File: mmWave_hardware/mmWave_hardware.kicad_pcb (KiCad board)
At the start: 6 copper layers, 50 x 21.6 mm, 48 parts, among them J1 Conn_02x08_Top_Bottom, U1 IWRL6432BDBAAMFR, U2 W25Q128JVS, U3 AMS1117-3.3, U4 TPS628502QDRLRQ1, Y1 40.000

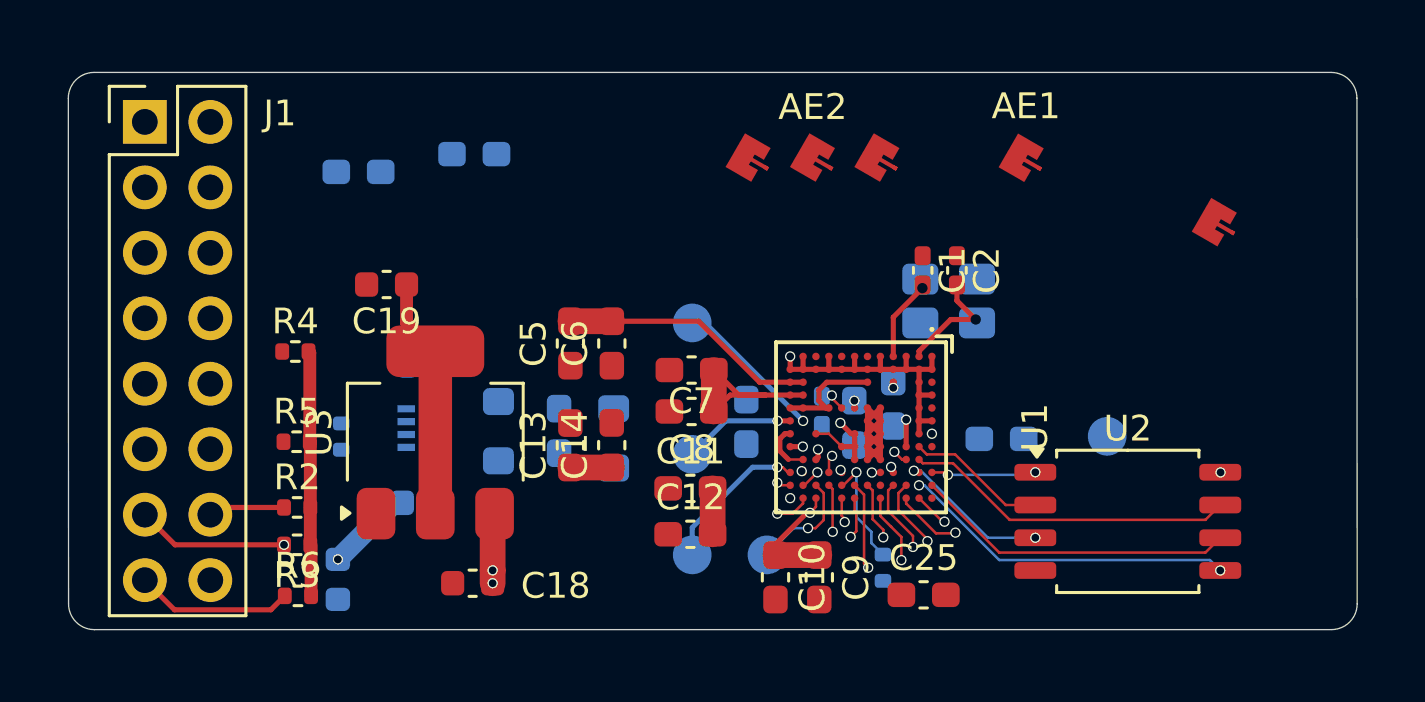
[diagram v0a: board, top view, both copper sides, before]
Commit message: PCB Complete
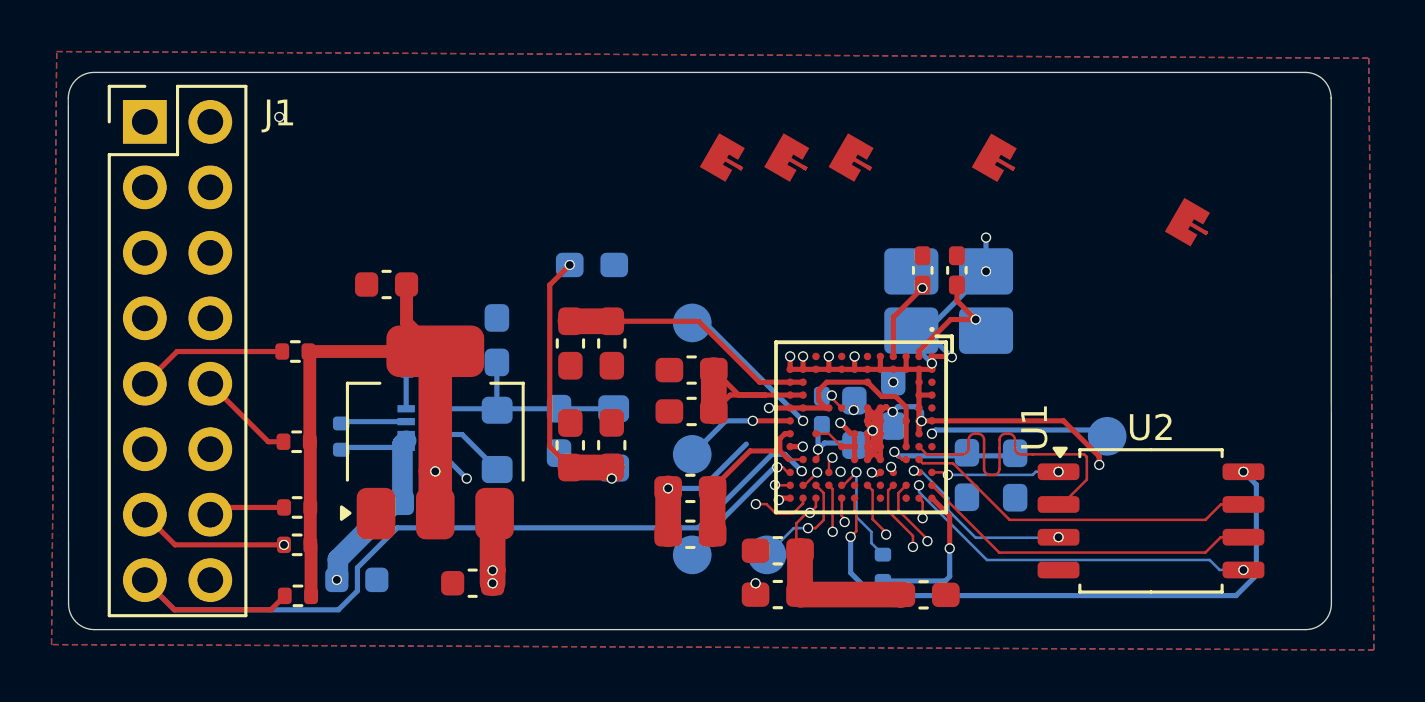
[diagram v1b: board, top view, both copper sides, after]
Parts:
- Y1: footprint Crystal:Crystal_SMD_3225-4Pin_3.2x2.5mm -> Crystal:Crystal_SMD_3225-4Pin_3.2x2.5mm_HandSoldering
- moved C3 8.80 mm to (83.9, 69.0)
- moved C24 8.45 mm to (65.6, 63.8), turned to 90 degrees
- moved C23 6.27 mm to (69.3, 60.9)
- moved C9 1.74 mm to (76.5, 73.6), turned to 180 degrees
- moved C4 1.52 mm to (85.7, 69.0), turned to -90 degrees
- moved AE1 1.04 mm to (84.9, 56.7)
- moved C10 1.03 mm to (76.5, 71.9), turned to 180 degrees
- moved AE2 1.00 mm to (76.9, 56.7)
- moved U2 0.90 mm to (91.0, 70.8)
- moved C20 0.74 mm to (60.2, 73.1), turned to 0 degrees
- moved L1 0.34 mm to (65.6, 67.6)
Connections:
- J1 pad 2: TCK -> GPIO_2
- J1 pad 3: TMS -> unconnected-(J1-Pin_3-Pad3)
- J1 pad 4: TDI -> GPIO_5
- J1 pad 5: TDO -> unconnected-(J1-Pin_5-Pad5)
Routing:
- net GND: track 23.6 -> 84.8 mm, vias 4 -> 20
- net RS232_RX: track 5.25 -> 51.0 mm
- net 3v3: track 21.0 -> 66.2 mm, vias 3 -> 4
- net GPIO_5: track 0.68 -> 41.8 mm
- net GPIO_2: track 0.14 -> 39.0 mm
- net UART_RTS: track 0.87 -> 36.3 mm
- net NRST_MAIN: track 6.13 -> 35.4 mm
- net 1v8: track 12.7 -> 41.0 mm, vias 3 -> 5
- net RS232_TX: track 30.4 -> 47.4 mm
- net Net-(U4-FB): track 0.00 -> 8.63 mm
- net /QSPI_1: track 5.50 -> 13.0 mm
- net Net-(U1-OSC_CLK_OUT): track 0.00 -> 6.96 mm
- net VIN: track 17.9 -> 23.0 mm
- net 1v2: track 6.57 -> 11.0 mm
- net SPI0_CLK: track 46.3 -> 50.5 mm
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- added copper zone on B.Cu, net GND
- added copper zone on F.Cu, net GND
- added copper zone on In1.Cu, net GND
- added copper zone on In2.Cu, net GND
- added copper zone on In3.Cu, net GND
- added copper zone on In4.Cu, net GND
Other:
- board size 50 x 21.6 mm -> 49 x 21.6 mm
